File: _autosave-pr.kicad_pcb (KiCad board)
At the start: 2 copper layers, 65 x 86 mm, 43 parts, among them P1 CONN_01X02, P2 CONN_01X02, P4 BDM, P5 CONN_01X03, P6 CONN_01X02, T1 TRANSFO, U1 78L05, U2 MC9S08SH8, U4 LM311N, U5 SSR_SHARP

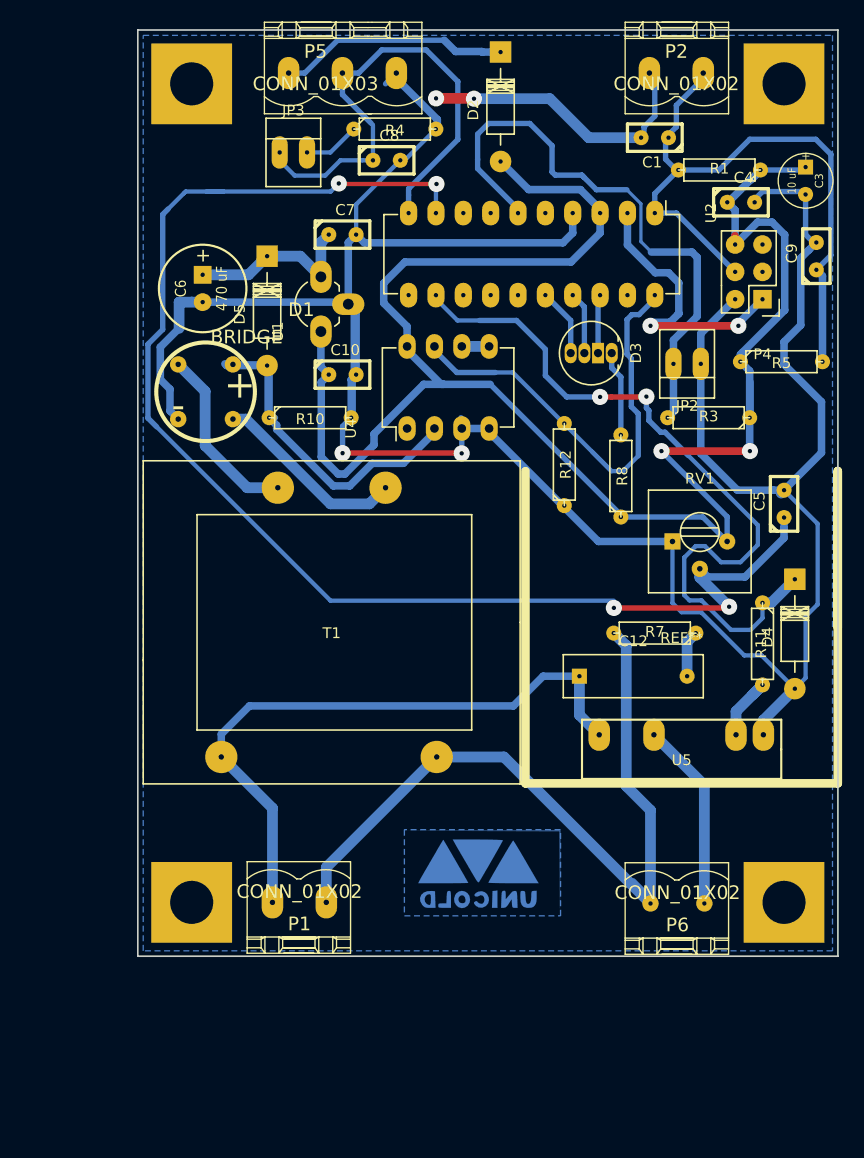
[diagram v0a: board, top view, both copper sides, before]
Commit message: modificado el esquematico
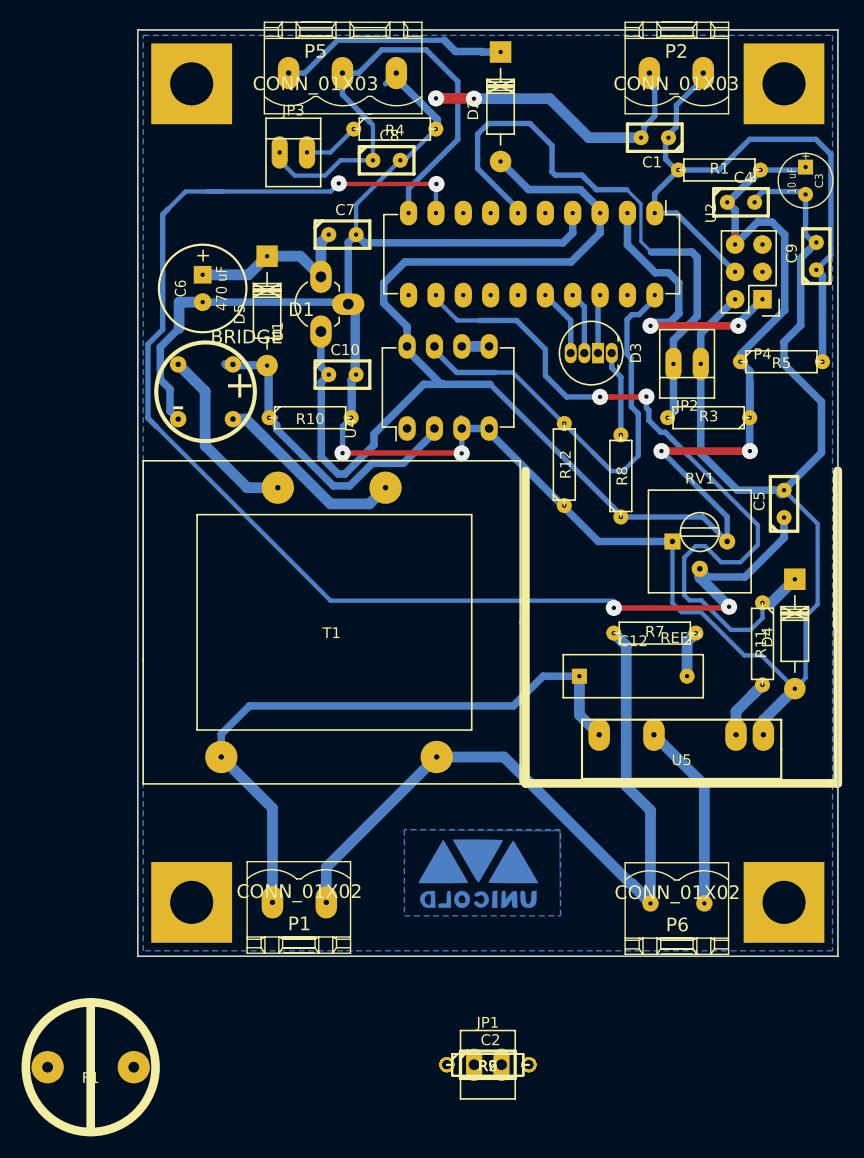
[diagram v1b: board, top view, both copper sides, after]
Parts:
- added C2: 0.1 uF, locales:C1, F.Cu at (76.5, 146.1)
- added F1: FUSE, locales:portafusible, F.Cu at (39.6, 146.3)
- added JP1: JUMPER, Connect:PINHEAD1-2, F.Cu at (76.5, 146.1)
- added R2, R6: 10k, Discret:R3, F.Cu at (76.5, 146.1)
- added R9: 390, Discret:R3, F.Cu at (76.5, 146.1)
- C8: value C -> 0,1 uF
- D2: value D -> 1N4007
- D4: value 1N4148 -> LED
- P2: value CONN_01X02 -> CONN_01X03
- R12: value 1M -> 1 M
- R3, R4: value R -> 10k
- R5: value 10K -> 10k
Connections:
- D1 pad 2: Net-(D1-Pad4) -> Net-(D1-Pad2)
- D1 pad 4: Net-(D1-Pad2) -> Net-(D1-Pad4)
- D4 pad 1: /AcOut -> Net-(D4-Pad1)
- D4 pad 2: GND -> Net-(C6-Pad1)
- D5 pad 1: Net-(C6-Pad1) -> /IZC
- D5 pad 2: /IZC -> Net-(C6-Pad1)
- P2 pad 2: /RESET -> /NM
- P6 pad 1: Net-(P6-Pad1) -> Net-(F1-Pad2)
- R12 pad 1: GND -> /ZC
- R12 pad 2: /ZC -> GND
- RV1 pad 1: GND -> /vreg
- RV1 pad 3: /vreg -> GND
- U1 pad 1: /vreg -> (no net)
- U1 pad 2: GND -> (no net)
- U1 pad 3: Net-(C6-Pad1) -> (no net)
- U2 pad 5: /GM -> /NM
- U5 pad 2: Net-(P6-Pad1) -> Net-(F1-Pad1)
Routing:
- net Net-(P6-Pad1): track 17.6 -> 0.00 mm
- net Net-(F1-Pad2): track 0.00 -> 11.0 mm
- net Net-(C6-Pad1): track 16.7 -> 27.5 mm
- net Net-(D1-Pad2): track 16.9 -> 24.3 mm
- net Net-(D1-Pad4): track 18.1 -> 10.7 mm
- net GND: track 288.0 -> 281.3 mm, vias 4 -> 5
- net Net-(F1-Pad1): track 0.00 -> 6.62 mm
- net /NM: track 0.00 -> 4.74 mm
- net /RESET: track 63.8 -> 59.1 mm
- net /IZC: track 39.9 -> 35.2 mm
- net Net-(D4-Pad1): track 0.00 -> 3.10 mm
- net /AcOut: track 75.4 -> 72.3 mm
- net /vreg: track 176.5 -> 177.0 mm, vias 2 -> 1
